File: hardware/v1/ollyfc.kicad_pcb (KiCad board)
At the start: 4 copper layers, 42.5 x 99.5 mm, 102 parts, among them J1 Conn_01x06, J10 Conn_01x03, J11 Conn_01x03, J12 Conn_01x04, J13 Conn_01x04, J14 Conn_01x04, J15 Conn_01x04, J2 Conn_01x02, J3 Conn_01x03, J4 USB_C_Receptacle_USB2.0, J5 Conn_02x05_Odd_Even, J6 Conn_01x03, J7 Conn_01x03, J8 Conn_Coaxial, J9 Conn_01x03, Q1 AO3401A, Q2 MMBT3904, Q3 MMBT3904, Q4 MMBT3904, SW2 SW_Push, SW3 SW_Push, SW4 MODE1, SW5 MODE1, U1 AMS1117-3.3, U10 SRV05-4, U2 PCA9685BS, U3 STM32F411RETx, U4 LIS3MDL, U5 BMI088, U6 W25Q128JVS, U7 BMP388, U8 NEO-M8N, U9 TPS2113APW, Y1 X322516MLB4SI

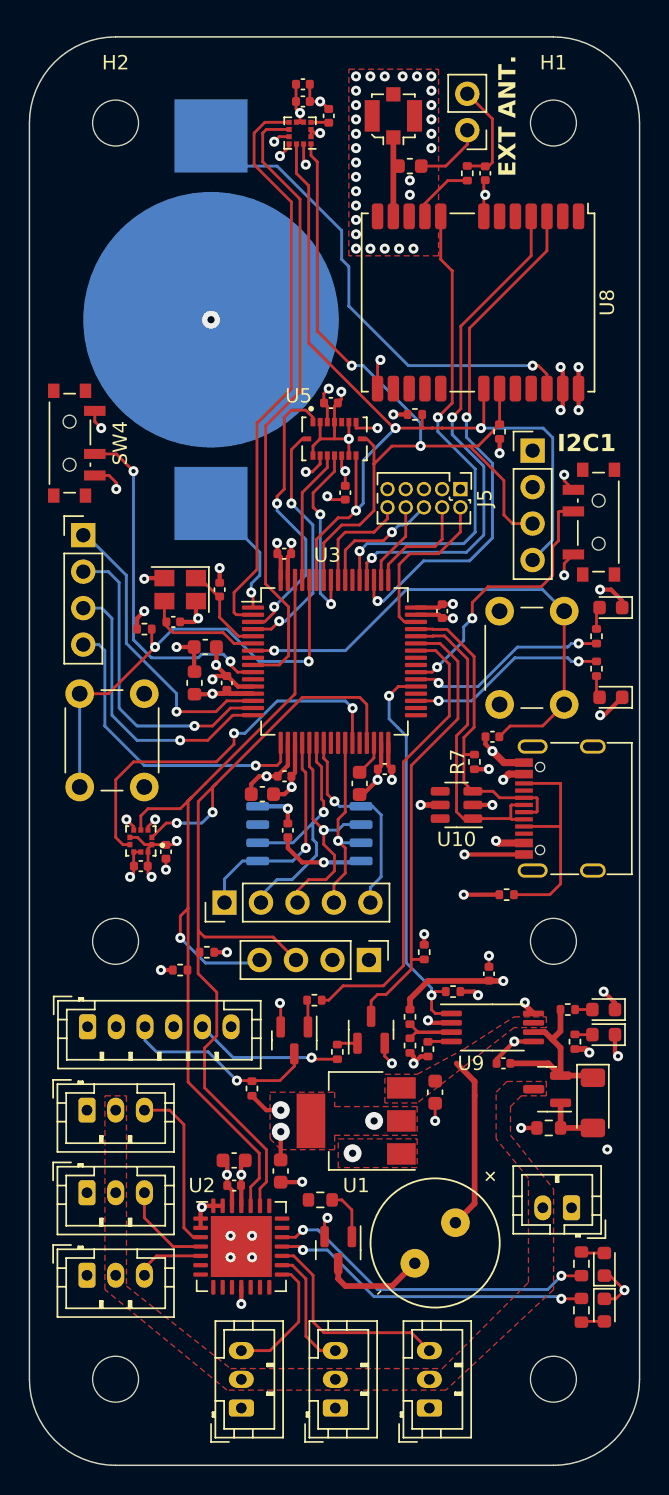
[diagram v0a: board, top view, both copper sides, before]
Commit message: v2 PCB design
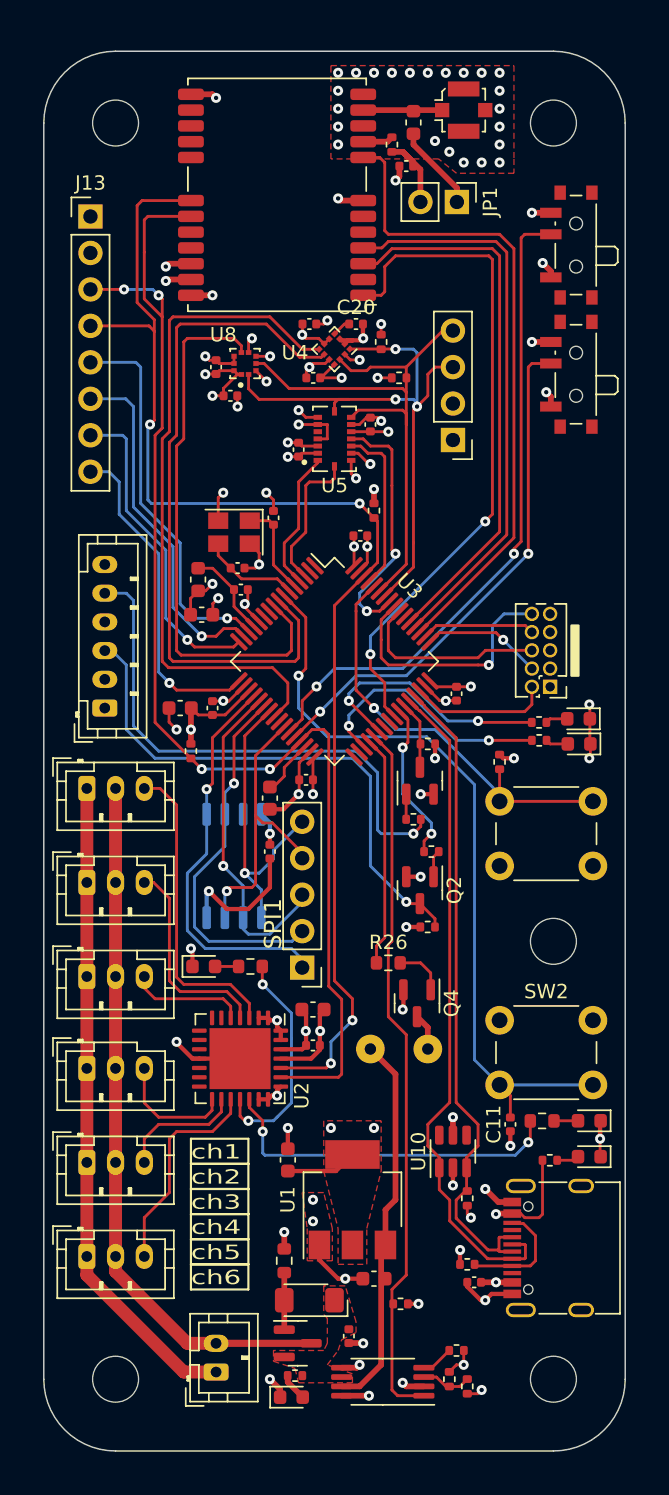
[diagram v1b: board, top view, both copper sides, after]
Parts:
- removed BT1: Battery_Cell, Battery:BatteryHolder_Keystone_3002_1x2032
- removed H6: MountingHole, MountingHole:MountingHole_3.2mm_M3
- removed J15: Conn_01x04, Connector_PinHeader_2.54mm:PinHeader_1x04_P2.54mm_Vertical
- BZ1: moved to B.Cu
- J13: footprint Connector_PinHeader_2.54mm:PinHeader_1x04_P2.54mm_Vertical -> Connector_PinHeader_2.54mm:PinHeader_1x08_P2.54mm_Vertical
- moved SW4 37.3 mm to (16.5, -29.0), turned to 90 degrees
- moved D4 36.8 mm to (-9.11, 21.2), turned to 0 degrees
- moved C15 35.2 mm to (-8.25, -20.5), turned to 90 degrees
- moved R8 34.7 mm to (2.75, -10.5), turned to -90 degrees
- moved D2 34.7 mm to (-3.00, 51.2), turned to 0 degrees
- moved U7 34.0 mm to (-6.24, -20.8), turned to 90 degrees
- moved R13 33.2 mm to (-5.86, 21.2), turned to 180 degrees
- moved C14 32.1 mm to (-7.25, -18.5), turned to 0 degrees
- moved R16 31.8 mm to (-2.75, 49.8), turned to 180 degrees
- moved J4 30.6 mm to (16.1, 40.9)
- moved H1 30.5 mm to (-15.2, -37.5)
- moved H2 30.5 mm to (15.2, -37.5)
- moved H5 30.5 mm to (15.2, 19.5)
- moved R7 30.4 mm to (9.25, 37.4)
- moved SW3 29.3 mm to (11.5, 9.75), turned to 0 degrees
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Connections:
- J13 pad 1: USART2_CTS -> GND
- J13 pad 2: USART2_RTS -> +3V3
- J13 pad 3: USART2_TX -> I2C2_SCL
- J13 pad 4: USART2_RX -> I2C2_SDA
- U3 pad 10: MODE1 -> unconnected-(U3-PC2-Pad10)
- U3 pad 2: MAG_INT -> unconnected-(U3-PC13-Pad2)
- U3 pad 24: unconnected-(U3-PC4-Pad24) -> MAG_INT
- U3 pad 27: PRES_INT -> MODE1
- U3 pad 28: unconnected-(U3-PB2-Pad28) -> MODE2
- U3 pad 3: ACCEL_INT2 -> ACCEL_INT1
- U3 pad 36: unconnected-(U3-PB15-Pad36) -> BUZZER
- U3 pad 39: MODE2 -> unconnected-(U3-PC8-Pad39)
- U3 pad 4: ACCEL_INT1 -> ACCEL_INT2
- U3 pad 41: unconnected-(U3-PA8-Pad41) -> GNSS_SAFEBOOT
- U3 pad 51: GNSS_TIMEP -> GNSS_RESET
- U3 pad 53: GNSS_RESET -> GNSS_TIMEP
- U3 pad 8: unconnected-(U3-PC0-Pad8) -> MAG_DRDY
- U3 pad 9: MAG_DRDY -> PRES_INT
- U7 pad 2: I2C2_SCL -> I2C1_SCL
- U7 pad 4: I2C2_SDA -> I2C1_SDA
- U8 pad 18: I2C1_SDA -> I2C2_SDA
- U8 pad 19: I2C1_SCL -> I2C2_SCL
- U8 pad 22: VBAT -> +3V3
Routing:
- net VIN_EXT: track 0.00 -> 49.3 mm
- net GNSS_SAFEBOOT: track 0.00 -> 47.3 mm, vias 0 -> 2
- net VBAT: track 43.0 -> 0.00 mm, vias 2 -> 0
- net GND: track 122.3 -> 156.2 mm, vias 86 -> 79
- net VBUS: track 14.9 -> 43.8 mm, vias 6 -> 5
- net I2C2_SDA: track 62.6 -> 90.1 mm, vias 1 -> 4
- net USART1_RX: track 31.9 -> 4.68 mm
- net /SBUS_OUT: track 10.3 -> 37.1 mm
- net I2C2_SCL: track 63.4 -> 88.7 mm, vias 2 -> 4
- net USBD-: track 22.0 -> 46.9 mm
- net /S_PORT: track 13.8 -> 37.6 mm
- net USBD+: track 22.1 -> 45.5 mm
- net I2C1_SDA: track 64.0 -> 41.9 mm, vias 3 -> 0
- net PWR_STATE: track 27.8 -> 49.4 mm, vias 2 -> 0
- net MODE1: track 24.6 -> 46.1 mm
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- added copper zone on F.Cu, net VIN
- removed copper zone on F.Cu, net 5VIN
- removed copper zone on In2.Cu, net VBUS
- removed copper zone on F.Cu, net VIN_EXT
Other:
- board size 42.5 x 99.5 mm -> 40.5 x 97.5 mm
- board text added: "SPI1"
- board text added: "ch1"
- board text added: "ch2"
- board text added: "ch3"
- board text added: "ch4"
- board text added: "ch5"
- board text added: "ch6"
- board text removed: "EXT ANT."
- board text removed: "I2C1"
